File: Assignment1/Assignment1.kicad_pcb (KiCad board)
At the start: 2 copper layers, 4 parts, among them SW1 SW_SPST

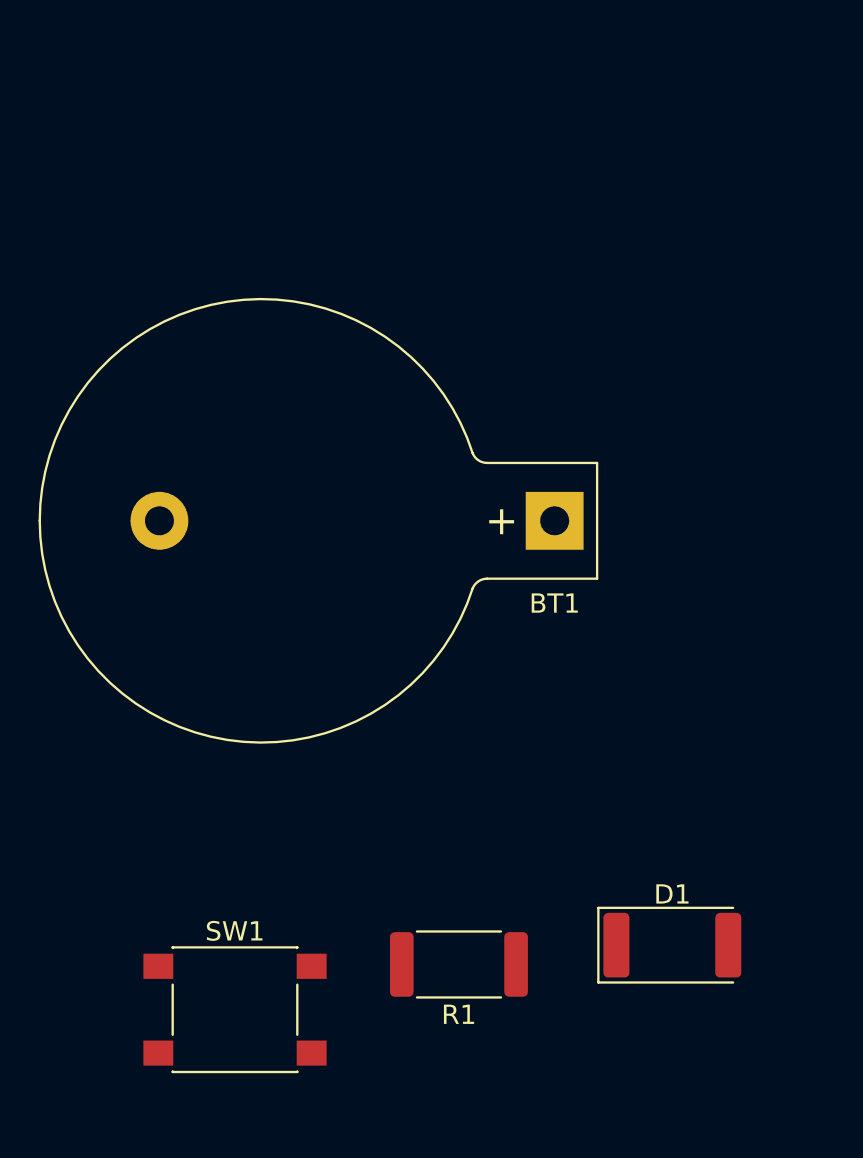
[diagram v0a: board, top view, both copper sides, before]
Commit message: All PNG files added
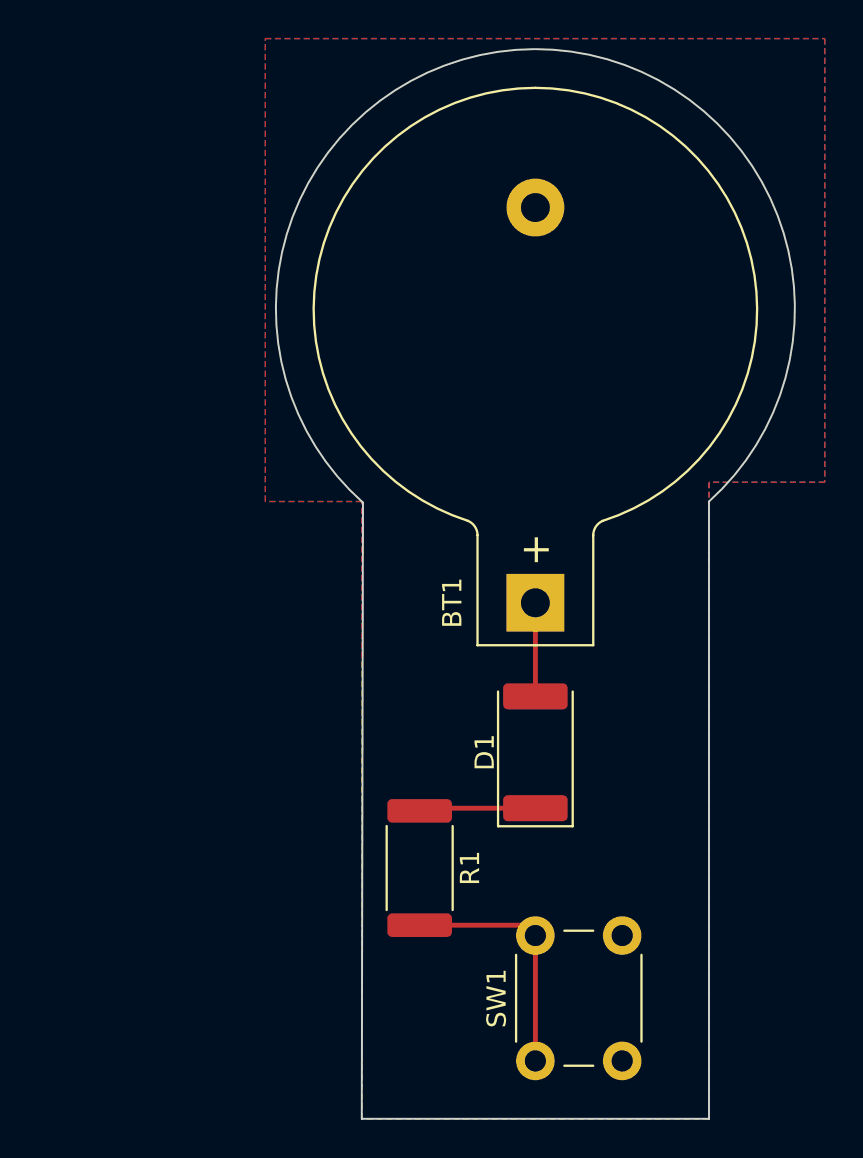
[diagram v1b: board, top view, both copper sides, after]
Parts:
- SW1: footprint Button_Switch_SMD:SW_Push_1P1T_NO_6x6mm_H9.5mm -> Button_Switch_THT:SW_PUSH_6mm
- moved SW1 15.8 mm to (99.0, 78.0), turned to 90 degrees
- moved D1 12.3 mm to (99.0, 62.0), turned to 90 degrees
- moved R1 5.40 mm to (93.0, 68.0), turned to -90 degrees
- moved BT1 4.37 mm to (99.0, 54.3), turned to 90 degrees
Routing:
- net Net-(SW1-A): track 0.00 -> 12.7 mm
- net Net-(D1-K): track 0.00 -> 6.06 mm
- net Net-(BT1-+): track 0.00 -> 4.85 mm
- added copper zone on B.Cu, net GND
- added copper zone on F.Cu, net GND
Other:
- board outline added: 26.9 x 55.5 mm
